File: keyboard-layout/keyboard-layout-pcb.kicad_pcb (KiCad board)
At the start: 2 copper layers, 205 parts, among them J1 USB_mini_micro_B, SW0 Undo, SW1 Redo, SW10 KEYSW, SW11 KEYSW, SW12 KEYSW, SW13 KEYSW, SW14 KEYSW, SW15 KEYSW, SW16 KEYSW, SW17 KEYSW, SW18 KEYSW, SW19 KEYSW, SW2 KEYSW, SW20 KEYSW, SW21 KEYSW, SW22 KEYSW, SW23 KEYSW, SW24 KEYSW, SW25 KEYSW, SW26 KEYSW, SW27 KEYSW, SW28 KEYSW, SW29 KEYSW, SW3 KEYSW, SW30 KEYSW, SW31 KEYSW, SW32 KEYSW, SW33 KEYSW, SW34 KEYSW, SW35 KEYSW, SW36 KEYSW, SW37 KEYSW, SW38 KEYSW, SW39 KEYSW, SW4 KEYSW, SW40 KEYSW, SW41 KEYSW, SW42 KEYSW, SW43 KEYSW, SW44 KEYSW, SW45 KEYSW, SW46 KEYSW, SW47 KEYSW, SW48 KEYSW, SW49 KEYSW, SW5 KEYSW, SW50 KEYSW, SW51 KEYSW, SW52 KEYSW, SW53 KEYSW, SW54 KEYSW, SW55 KEYSW, SW56 KEYSW, SW57 KEYSW, SW58 KEYSW, SW59 KEYSW, SW6 KEYSW, SW60 KEYSW, SW61 KEYSW, SW62 KEYSW, SW63 KEYSW, SW64 KEYSW, SW65 KEYSW, SW66 KEYSW, SW67 KEYSW, SW68 KEYSW, SW69 KEYSW, SW7 KEYSW, SW70 KEYSW, SW71 KEYSW, SW72 KEYSW, SW73 KEYSW, SW74 KEYSW, SW75 KEYSW, SW76 KEYSW, SW77 KEYSW, SW78 KEYSW, SW79 KEYSW, SW8 KEYSW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

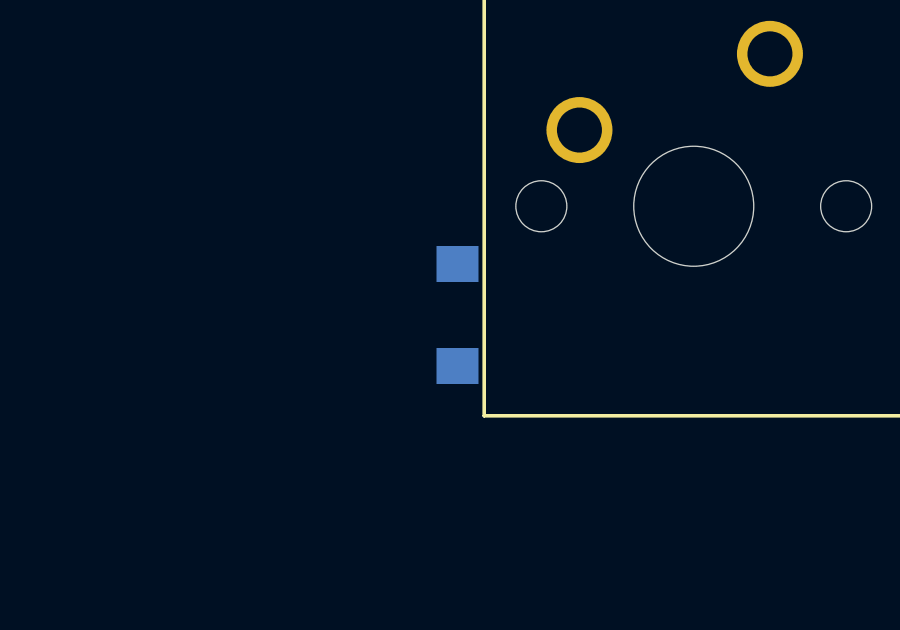
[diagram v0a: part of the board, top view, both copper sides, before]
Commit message: Bitz
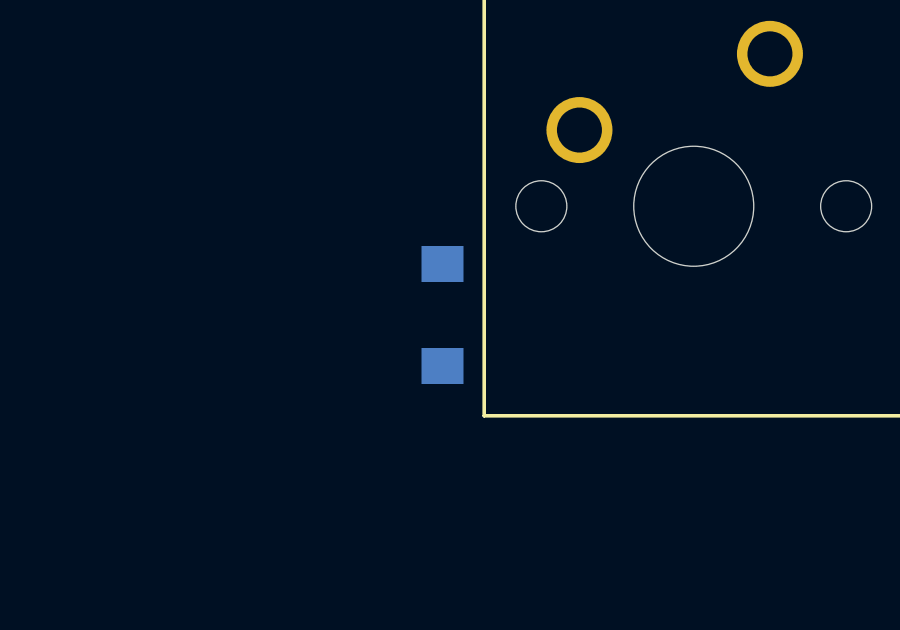
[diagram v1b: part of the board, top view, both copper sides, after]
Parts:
- moved D0 0.50 mm to (136.5, 63.0)
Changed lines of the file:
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@@
     (links 328)
     (no_connects 230)
-    (area -21.864 -14.950001 449.815 169.565)
+    (area -21.864 -6.26 449.815 169.565)
     (thickness 1.6)
     (drawings 0)
@@
   )
   (module keyboard_parts:D_SOD123W_hand (layer B.Cu)
-    (at 137 63 90)
+    (at 136.5 63 90)
     (attr smd)
     (fp_text reference D0 (at 0 -1.925 90) (layer B.SilkS)
